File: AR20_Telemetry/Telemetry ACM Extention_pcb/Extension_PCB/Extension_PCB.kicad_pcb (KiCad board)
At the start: 2 copper layers, 2 parts, among them U1 ACM_2020

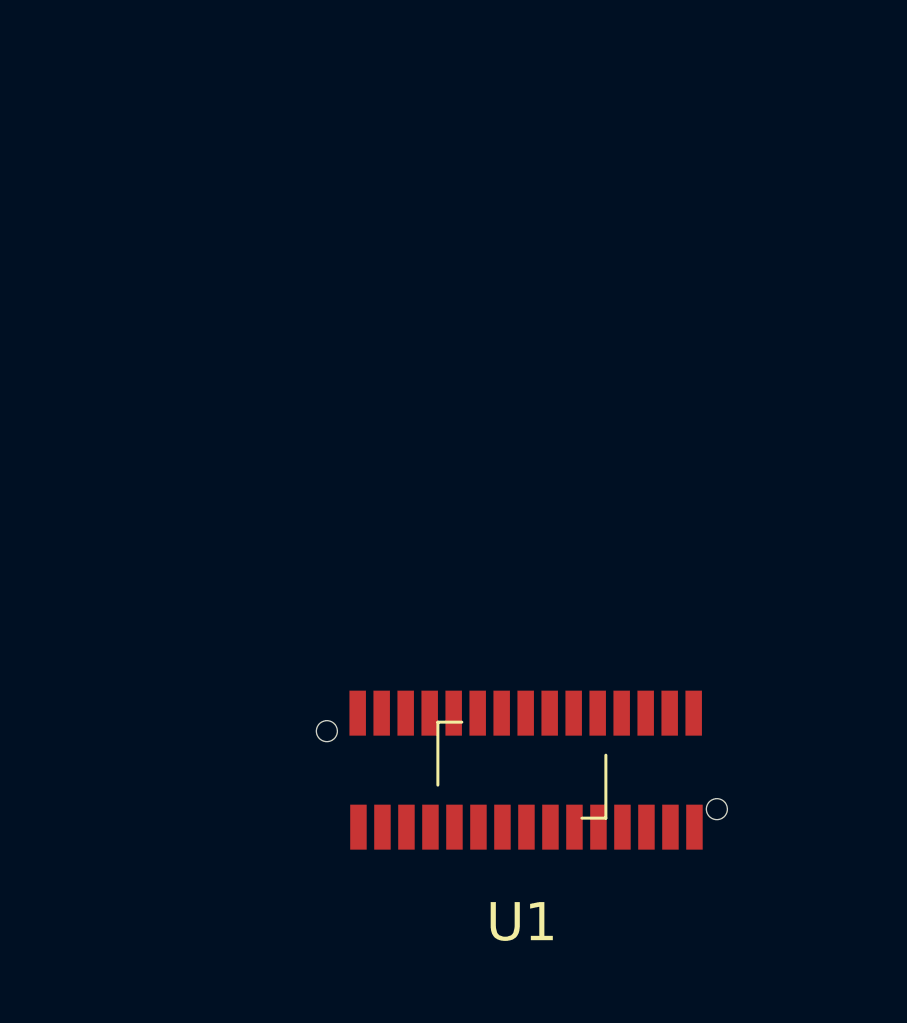
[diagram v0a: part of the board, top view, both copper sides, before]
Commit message: Edited
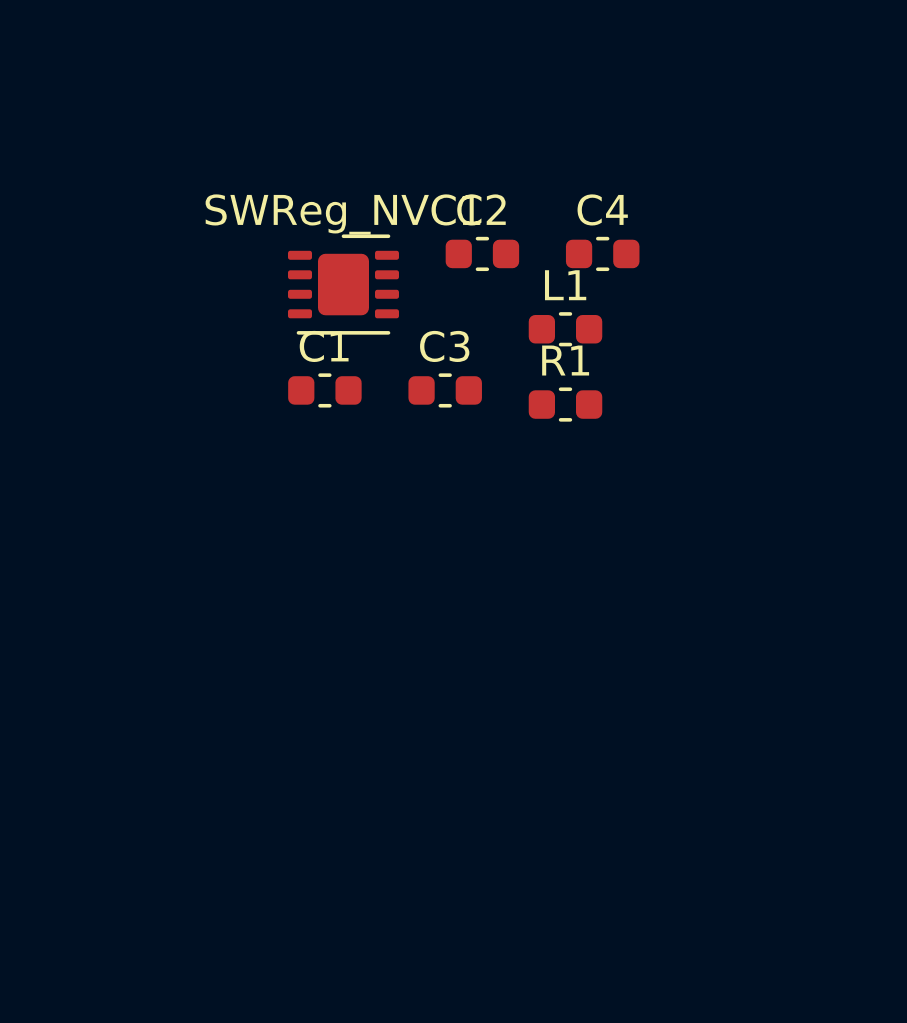
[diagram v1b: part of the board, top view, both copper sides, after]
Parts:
- removed U1: ACM_2020, MCP25625_Breakoutboard:ACM_2020_Footprint
- added C1: 10u, Capacitor_SMD:C_0603_1608Metric, F.Cu at (166.4, 129.6)
- added C2: 0.1u, Capacitor_SMD:C_0603_1608Metric, F.Cu at (171.6, 125.0)
- added C3: 0.1u, Capacitor_SMD:C_0603_1608Metric, F.Cu at (170.4, 129.6)
- added C4: 10u, Capacitor_SMD:C_0603_1608Metric, F.Cu at (175.6, 125.0)
- added L1: 2.2u, Inductor_SMD:L_0603_1608Metric, F.Cu at (174.4, 127.5)
- added R1: 10k, Resistor_SMD:R_0603_1608Metric, F.Cu at (174.4, 130.1)
- added SWReg_NVC1: NCV890430MW50TXG, Package_DFN_QFN:DFN-8-1EP_3x3mm_P0.65mm_EP1.7x2.05mm, F.Cu at (167.0, 126.1)
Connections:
- A1 pad 29: (no net) -> Ground
- A1 pad 6: (no net) -> Ground
- A1 pad 7: (no net) -> Ground
- A1 pad 8: (no net) -> Ground
